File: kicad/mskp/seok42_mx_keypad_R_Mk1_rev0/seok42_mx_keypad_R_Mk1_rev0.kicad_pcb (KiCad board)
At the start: 2 copper layers, 142 x 102 mm, 50 parts, among them J1 Conn_01x12_Socket, SW1 Switch, SW10 Switch, SW11 Switch, SW12 Switch, SW13 Switch, SW14 Switch, SW15 Switch, SW16 Switch, SW17 Switch, SW18 Switch, SW19 Switch, SW2 Switch, SW20 Switch, SW21 Switch, SW3 Switch, SW4 Switch, SW5 Switch, SW6 Switch, SW7 Switch, SW8 Switch, SW9 Switch

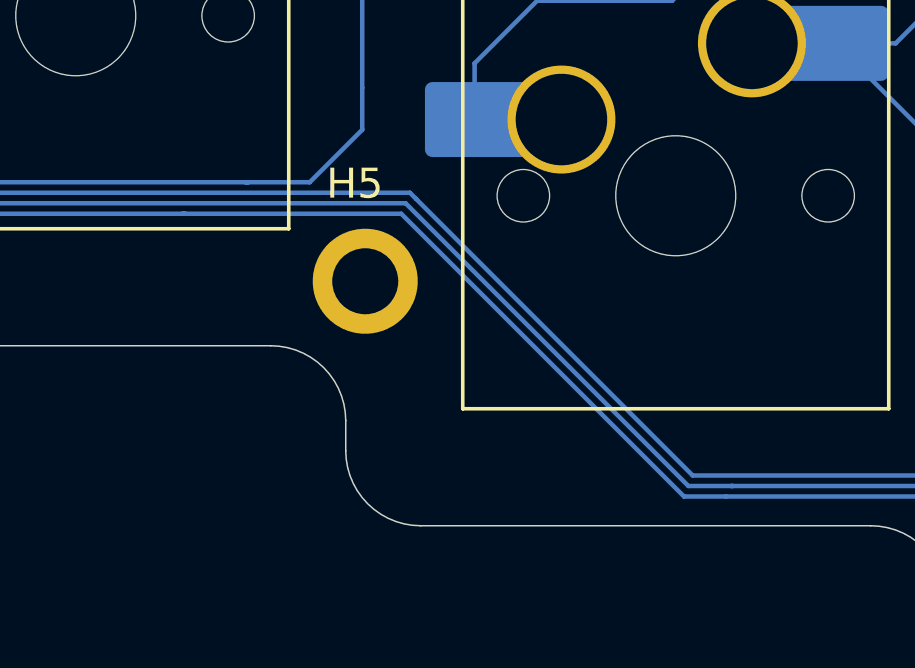
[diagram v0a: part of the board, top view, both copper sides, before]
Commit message: Final tweaks to PCBs before second round of mskp fabrications
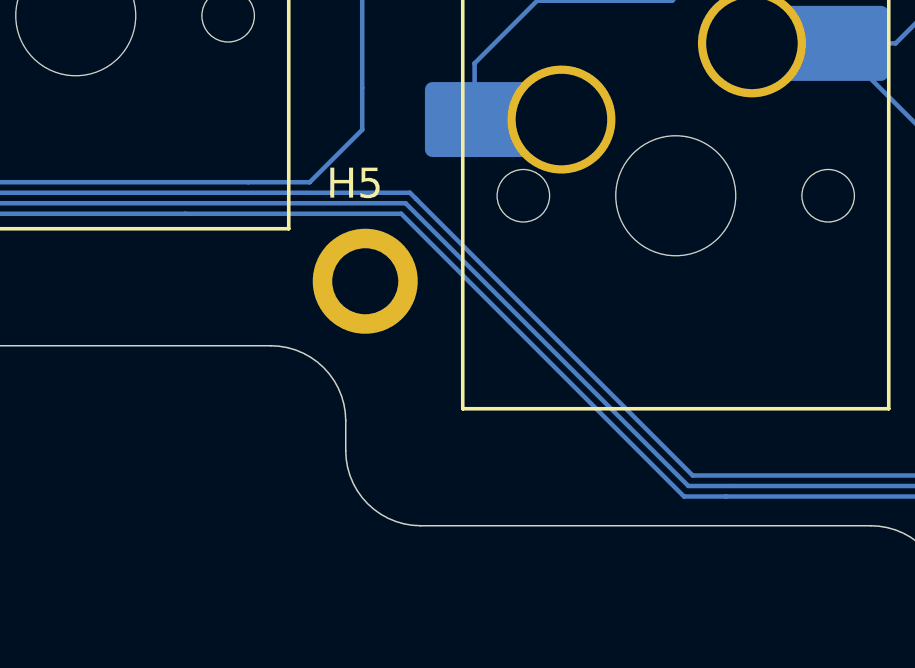
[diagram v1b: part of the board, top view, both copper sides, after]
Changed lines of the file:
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@@
 			(plot_on_all_layers_selection 0x0000000_00000000)
 			(disableapertmacros no)
-			(usegerberextensions no)
-			(usegerberattributes yes)
-			(usegerberadvancedattributes yes)
-			(creategerberjobfile yes)
+			(usegerberextensions yes)
+			(usegerberattributes no)
+			(usegerberadvancedattributes no)
+			(creategerberjobfile no)
 			(dashed_line_dash_ratio 12.000000)
 			(dashed_line_gap_ratio 3.000000)
 			(svgprecision 4)
 			(plotframeref no)
-			(viasonmask no)
+			(viasonmask yes)
 			(mode 1)
 			(useauxorigin no)
@@
 			(psa4output no)
 			(plotreference yes)
-			(plotvalue yes)
+			(plotvalue no)
 			(plotfptext yes)
 			(plotinvisibletext no)
 			(sketchpadsonfab no)
-			(subtractmaskfromsilk no)
+			(subtractmaskfromsilk yes)
 			(outputformat 1)
 			(mirror no)
-			(drillshape 1)
+			(drillshape 0)
 			(scaleselection 1)
-			(outputdirectory "")
+			(outputdirectory "seok42_r_mk1_exports")
 		)
 	)
@@
 	)
 	(segment
-		(start 159.75 98.55)
-		(end 159.65 98.55)
-		(width 0.15)
-		(layer "B.Cu")
-		(net 25)
-	)
-	(segment
 		(start 140.4 107.35)
 		(end 123.215076 107.35)
@@
 	)
 	(segment
-		(start 157.65 99.6)
-		(end 157.55 99.6)
-		(width 0.15)
-		(layer "B.Cu")
-		(net 28)
-	)
-	(segment
 		(start 221.85 111.45)
 		(end 221.85 116.3)
@@
 		(width 0.15)
 		(layer "B.Cu")
-		(net 29)
-	)
-	(segment
-		(start 175.9 108.675)
-		(end 175.825 108.675)
-		(width 0.15)
-		(layer "B.Cu")
